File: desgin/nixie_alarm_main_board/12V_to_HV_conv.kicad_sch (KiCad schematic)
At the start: 21 parts, among them IC1 LM3488MM, IC8 MCP4018T-502E_LT, Q9 TPH5200FNH,L1Q

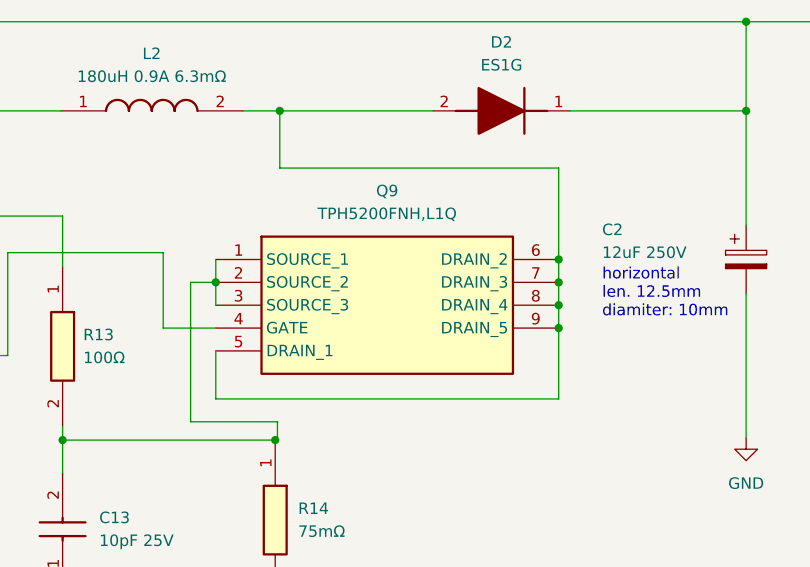
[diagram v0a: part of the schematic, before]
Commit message: new layout
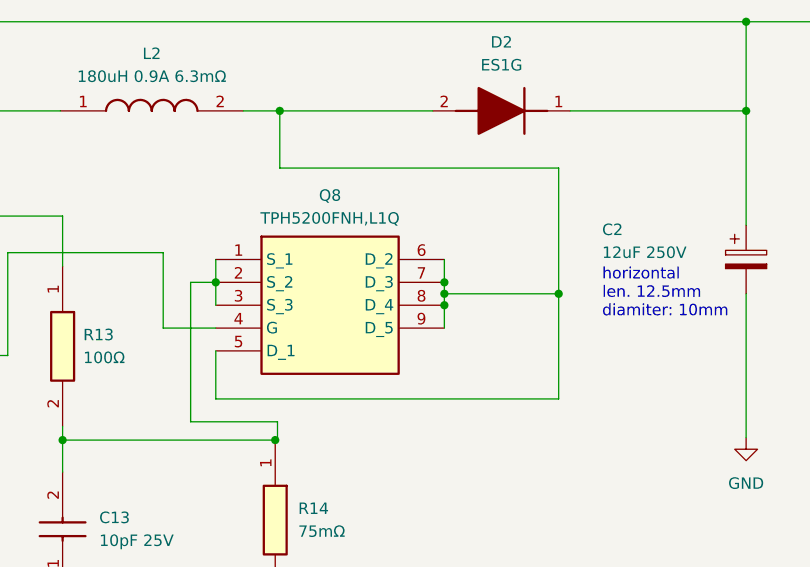
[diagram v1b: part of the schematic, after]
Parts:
- removed Q9: TPH5200FNH,L1Q, Package_SO:SO-8_3.9x4.9mm_P1.27mm, symbol SamacSys_Parts:TPH1110FNH,L1Q
- added Q8: TPH5200FNH,L1Q, TPHR6503PL1LQ, symbol SamacSys_Parts:TPHR6503PL1,LQ
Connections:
- net at D2.2 (A), L2.2: now also Q8.5 (D_1), Q8.6 (D_2), Q8.7 (D_3), Q8.8 (D_4), Q8.9 (D_5)
- net at C13.2, R13.2, R14.1: now also Q8.1 (S_1), Q8.2 (S_2), Q8.3 (S_3)
- net at IC1.6 (DR): now also Q8.4 (G)

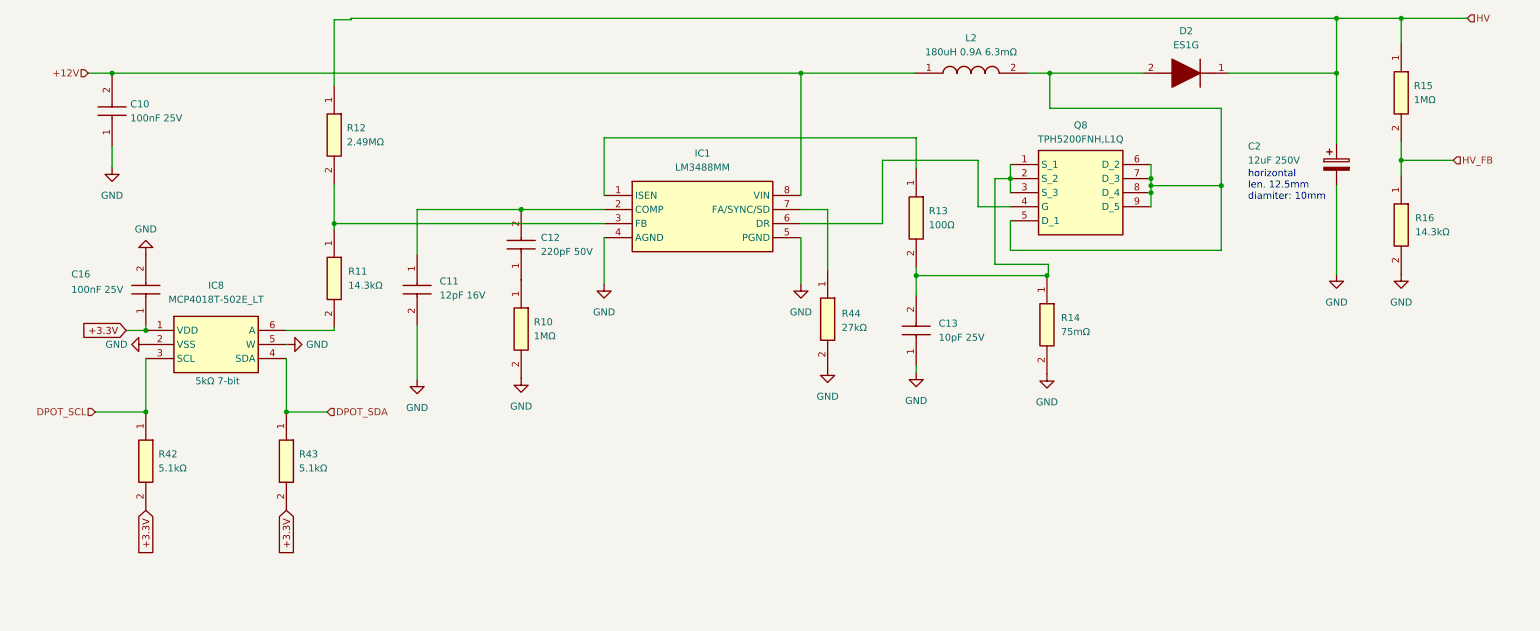
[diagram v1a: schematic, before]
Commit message: fixes added
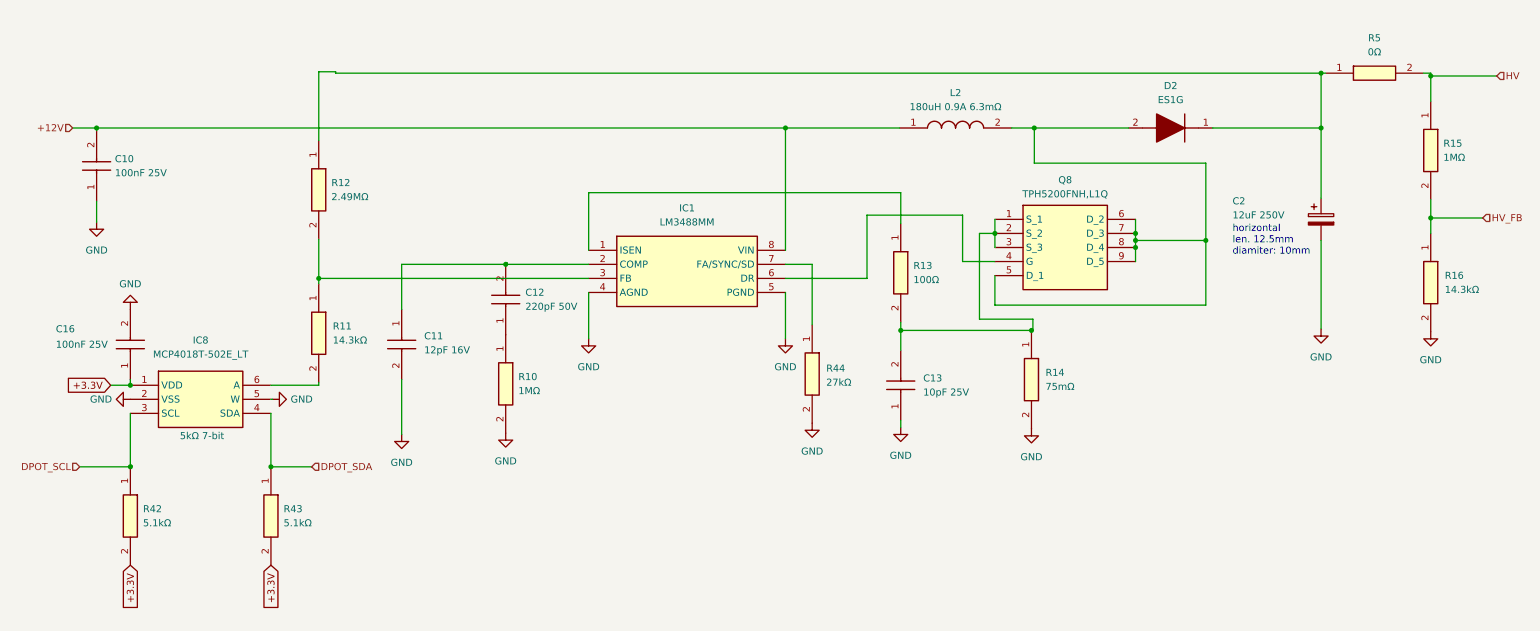
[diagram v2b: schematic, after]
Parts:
- added R5: 0Ω, Resistor_SMD:R_0805_2012Metric_Pad1.20x1.40mm_HandSolder, symbol SamacSys_Parts:CRCW04022K74FKED
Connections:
- net HV: now also R5.2; no longer C2.1, D2.1 (K), R12.1
- new net: C2.1, D2.1 (K), R12.1, R5.1
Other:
- moved on the sheet: C10, C11, C12, C13, C16, C2, D2, IC1, IC8, L2, Q8, R10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
